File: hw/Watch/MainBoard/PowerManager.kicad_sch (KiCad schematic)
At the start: 4 parts, among them U4 LD39200

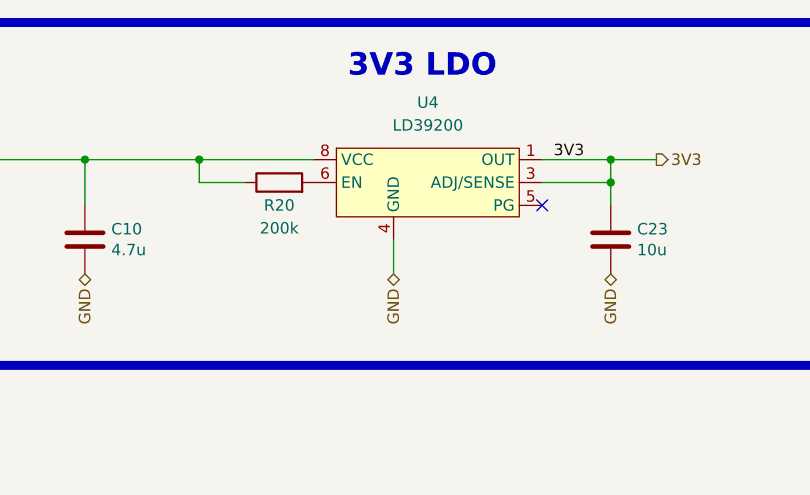
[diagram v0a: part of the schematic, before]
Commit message: wip
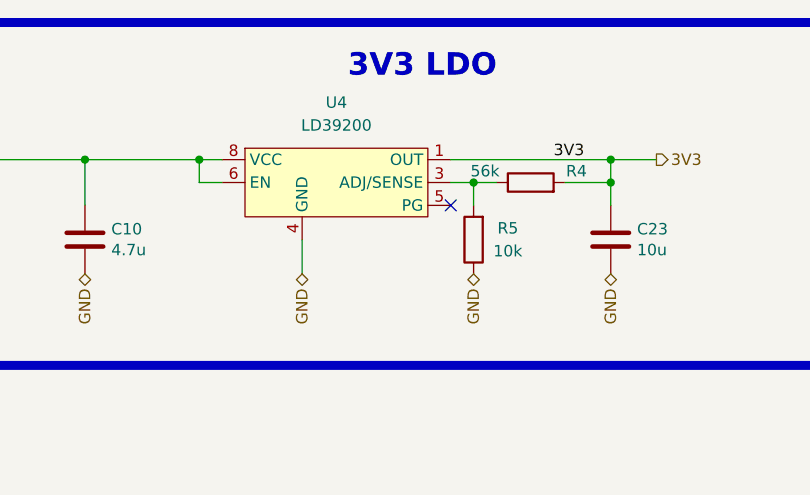
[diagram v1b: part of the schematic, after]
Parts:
- removed R20: 200k, Resistor_SMD:R_0402_1005Metric, symbol Device:R
- added R4: 56k, Resistor_SMD:R_0402_1005Metric, symbol Device:R
- added R5: 10k, Resistor_SMD:R_0201_0603Metric, symbol Device:R
- C10: footprint Capacitor_SMD:C_0603_1608Metric -> Capacitor_SMD:C_0402_1005Metric; LCSC C19666 -> C23733
- C23: footprint Capacitor_SMD:C_0603_1608Metric -> Capacitor_SMD:C_0402_1005Metric; Basic/Extended B -> E; LCSC C96446 -> C315248; info 25V, X5R -> 10V, X5R
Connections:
- net 3V3: now also R4.2; no longer U4.3 (ADJ/SENSE)
- net GND: now also R5.1
- net VCC: now also U4.6 (EN)
- new net: R4.1, R5.2, U4.3 (ADJ/SENSE)
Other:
- moved on the sheet: U4
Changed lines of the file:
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@@
   (junction (at 152.4 40.64) (diameter 0) (color 0 0 0 0)
   )
+  (junction (at 195.58 43.18) (diameter 0) (color 0 0 0 0)
+  )
   (junction (at 210.82 40.64) (diameter 0) (color 0 0 0 0)
   )
@@
   )
   (no_connect (at 137.16 129.54))
-  (no_connect (at 203.2 45.72))
+  (no_connect (at 193.04 45.72))
   (no_connect (at 137.16 127))
   (wire (pts (xy 210.82 43.18) (xy 210.82 40.64))
@@
     (stroke (width 0) (type default))
   )
-  (wire (pts (xy 203.2 40.64) (xy 210.82 40.64))
+  (wire (pts (xy 193.04 40.64) (xy 210.82 40.64))
+    (stroke (width 0) (type default))
+  )
+  (wire (pts (xy 195.58 43.18) (xy 198.12 43.18))
+    (stroke (width 0) (type default))
+  )
+  (wire (pts (xy 195.58 43.18) (xy 195.58 45.72))
     (stroke (width 0) (type default))
   )
@@
     (stroke (width 1) (type default))
   )
-  (wire (pts (xy 165.1 40.64) (xy 177.8 40.64))
+  (wire (pts (xy 165.1 40.64) (xy 167.64 40.64))
     (stroke (width 0) (type default))
   )
@@
     (stroke (width 0) (type default))
   )
-  (wire (pts (xy 186.69 49.53) (xy 186.69 53.34))
+  (wire (pts (xy 176.53 49.53) (xy 176.53 53.34))
     (stroke (width 0) (type default))
   )
@@
     (stroke (width 0) (type default))
   )
-  (wire (pts (xy 203.2 43.18) (xy 210.82 43.18))
-    (stroke (width 0) (type default))
-  )
-  (wire (pts (xy 170.18 43.18) (xy 165.1 43.18))
+  (wire (pts (xy 193.04 43.18) (xy 195.58 43.18))
+    (stroke (width 0) (type default))
+  )
+  (wire (pts (xy 165.1 43.18) (xy 167.64 43.18))
     (stroke (width 0) (type default))
   )
@@
   )
   (wire (pts (xy 104.14 73.66) (xy 101.6 73.66))
+    (stroke (width 0) (type default))
+  )
+  (wire (pts (xy 205.74 43.18) (xy 210.82 43.18))
     (stroke (width 0) (type default))
   )
@@
     (effects (font (size 1.27 1.27)) (justify left bottom))
   )
+  (hierarchical_label "GND" (shape bidirectional) (at 195.58 53.34 270) (fields_autoplaced)
+    (effects (font (size 1.27 1.27)) (justify right))
+  )
   (hierarchical_label "3V3" (shape output) (at 215.9 40.64 0) (fields_autoplaced)
     (effects (font (size 1.27 1.27)) (justify left))
@@
     (effects (font (size 1.27 1.27)) (justify right))
   )
-  (hierarchical_label "GND" (shape bidirectional) (at 186.69 53.34 270) (fields_autoplaced)
+  (hierarchical_label "GND" (shape bidirectional) (at 176.53 53.34 270) (fields_autoplaced)
     (effects (font (size 1.27 1.27)) (justify right))
   )
@@
       (effects (font (size 1.27 1.27)) (justify left))
     )
-    (property "Footprint" "Capacitor_SMD:C_0603_1608Metric" (at 211.7852 53.34 0)
+    (property "Footprint" "Capacitor_SMD:C_0402_1005Metric" (at 211.7852 53.34 0)
       (effects (font (size 1.27 1.27)) hide)
     )
@@
       (effects (font (size 1.27 1.27)) hide)
     )
-    (property "LCSC" "C96446" (at 210.82 49.53 0)
-      (effects (font (size 1.27 1.27)) hide)
-    )
-    (property "Basic/Extended" "B" (at 210.82 49.53 0)
-      (effects (font (size 1.27 1.27)) hide)
-    )
-    (property "info" "25V, X5R" (at 210.82 49.53 0)
+    (property "LCSC" "C315248" (at 210.82 49.53 0)
+      (effects (font (size 1.27 1.27)) hide)
+    )
+    (property "Basic/Extended" "E" (at 210.82 49.53 0)
+      (effects (font (size 1.27 1.27)) hide)
+    )
+    (property "info" "10V, X5R" (at 210.82 49.53 0)
       (effects (font (size 1.27 1.27)) hide)
     )
@@
       (effects (font (size 1.27 1.27)) (justify left))
     )
-    (property "Footprint" "Capacitor_SMD:C_0603_1608Metric" (at 153.3652 53.34 0)
+    (property "Footprint" "Capacitor_SMD:C_0402_1005Metric" (at 153.3652 53.34 0)
       (effects (font (size 1.27 1.27)) hide)
     )
@@
       (effects (font (size 1.27 1.27)) hide)
     )
-    (property "LCSC" "C19666" (at 152.4 49.53 0)
+    (property "LCSC" "C23733" (at 152.4 49.53 0)
       (effects (font (size 1.27 1.27)) hide)
     )
@@
     )
   )
-  (symbol (lib_id "Device:R") (at 173.99 43.18 90) (unit 1)
+  (symbol (lib_id "Device:R") (at 201.93 43.18 90) (unit 1)
     (in_bom yes) (on_board yes) (dnp no)
-    (property "Reference" "R20" (at 173.99 45.72 90)
-      (effects (font (size 1.27 1.27)))
-    )
-    (property "Value" "200k" (at 173.99 48.26 90)
-      (effects (font (size 1.27 1.27)))
-    )
-    (property "Footprint" "Resistor_SMD:R_0402_1005Metric" (at 173.99 44.958 90)
-      (effects (font (size 1.27 1.27)) hide)
-    )
-    (property "Datasheet" "~" (at 173.99 43.18 0)
-      (effects (font (size 1.27 1.27)) hide)
-    )
-    (property "LCSC" "C25764" (at 173.99 43.18 0)
-      (effects (font (size 1.27 1.27)) hide)
-    )
-    (property "Basic/Extended" "B" (at 173.99 43.18 0)
+    (property "Reference" "R4" (at 207.01 41.91 90)
+      (effects (font (size 1.27 1.27)))
+    )
+    (property "Value" "56k" (at 196.85 41.91 90)
+      (effects (font (size 1.27 1.27)))
+    )
+    (property "Footprint" "Resistor_SMD:R_0402_1005Metric" (at 201.93 44.958 90)
+      (effects (font (size 1.27 1.27)) hide)
+    )
+    (property "Datasheet" "~" (at 201.93 43.18 0)
+      (effects (font (size 1.27 1.27)) hide)
+    )
+    (property "LCSC" "C25796" (at 201.93 43.18 0)
       (effects (font (size 1.27 1.27)) hide)
     )
@@
       (project "Watch"
         (path "/1db6f6a7-b341-422f-8dcc-b4fd8e3ba0c0/7a0b441f-fb08-4406-ad74-ba91736d76e3/e51762e8-40da-4e3a-afe4-857a6428bc26"
-          (reference "R20") (unit 1)
-        )
-      )
-      (project "ZakladniElektronika"
-        (path "/99cd3e15-4eb6-4cbb-8726-789aedd3df15/c3b70d9b-0dcb-4344-9507-13ff5b4c000e/aae02708-da26-44dd-a602-660fbe003309/3940fef8-969a-4db4-8b0b-434b96d98566"
-          (reference "R50") (unit 1)
-        )
-      )
-      (project "RB3203"
-        (path "/dc7f8a41-3453-4df6-94dc-e94521e89591/9c917b4f-c6c7-4191-9aaa-f982c264da50/8773969d-b2cc-42c4-9a6d-35c6f165cf16/da5be375-027b-4f55-96f0-042c23671c4c"
-          (reference "U?") (unit 1)
-        )
-      )
-    )
-  )
-  (symbol (lib_id "RKL-LDO:LD39200") (at 190.5 40.64 0) (unit 1)
+          (reference "R4") (unit 1)
+        )
+      )
+      (project "SemiSemafor"
+        (path "/fb82d987-26cf-425e-8e99-22ecb59c8a96"
+          (reference "R11") (unit 1)
+        )
+      )
+    )
+  )
+  (symbol (lib_id "Device:R") (at 195.58 49.53 180) (unit 1)
+    (in_bom yes) (on_board yes) (dnp no)
+    (property "Reference" "R5" (at 199.39 48.26 0)
+      (effects (font (size 1.27 1.27)))
+    )
+    (property "Value" "10k" (at 199.39 50.8 0)
+      (effects (font (size 1.27 1.27)))
+    )
+    (property "Footprint" "Resistor_SMD:R_0201_0603Metric" (at 197.358 49.53 90)
+      (effects (font (size 1.27 1.27)) hide)
+    )
+    (property "Datasheet" "~" (at 195.58 49.53 0)
+      (effects (font (size 1.27 1.27)) hide)
+    )
+    (property "LCSC" "C106225" (at 195.58 49.53 0)
+      (effects (font (size 1.27 1.27)) hide)
+    )
+    (property "Basic/Extended" "E" (at 195.58 49.53 0)
+      (effects (font (size 1.27 1.27)) hide)
+    )
+    (pin "1")
+    (pin "2")
+    (instances
+      (project "Watch"
+        (path "/1db6f6a7-b341-422f-8dcc-b4fd8e3ba0c0/7a0b441f-fb08-4406-ad74-ba91736d76e3/e51762e8-40da-4e3a-afe4-857a6428bc26"
+          (reference "R5") (unit 1)
+        )
+      )
+      (project "SemiSemafor"
+        (path "/fb82d987-26cf-425e-8e99-22ecb59c8a96"
+          (reference "R10") (unit 1)
+        )
+      )
+    )
+  )
+  (symbol (lib_id "RKL-LDO:LD39200") (at 180.34 40.64 0) (unit 1)
     (in_bom yes) (on_board yes) (dnp no) (fields_autoplaced)
-    (property "Reference" "U4" (at 190.5 34.29 0)
-      (effects (font (size 1.27 1.27)))
-    )
-    (property "Value" "LD39200" (at 190.5 36.83 0)
-      (effects (font (size 1.27 1.27)))
-    )
-    (property "Footprint" "Package_DFN_QFN:DFN-8-1EP_4x4mm_P0.8mm_EP2.3x3.24mm" (at 190.5 33.02 0)
-      (effects (font (size 1.27 1.27)) hide)
-    )
-    (property "Datasheet" "https://datasheet.lcsc.com/lcsc/2010270935_STMicroelectronics-LD39200DPUR_C880590.pdf" (at 190.5 30.48 0)
-      (effects (font (size 1.27 1.27)) hide)
-    )
-    (property "LCSC" "C880590" (at 190.5 27.94 0)
-      (effects (font (size 1.27 1.27)) hide)
-    )
-    (property "Basic/Extended" "E" (at 190.5 40.64 0)
-      (effects (font (size 1.27 1.27)) hide)
-    )
-    (property "JLCPCB_CORRECTION" "0;0;-90" (at 190.5 40.64 0)
-      (effects (font (size 1.27 1.27)) hide)
-    )
+    (property "Reference" "U4" (at 180.34 34.29 0)
+      (effects (font (size 1.27 1.27)))
+    )
+    (property "Value" "LD39200" (at 180.34 36.83 0)
+      (effects (font (size 1.27 1.27)))
+    )
+    (property "Footprint" "Package_DFN_QFN:DFN-8-1EP_4x4mm_P0.8mm_EP2.3x3.24mm" (at 180.34 33.02 0)
+      (effects (font (size 1.27 1.27)) hide)
+    )
+    (property "Datasheet" "https://datasheet.lcsc.com/lcsc/2010270935_STMicroelectronics-LD39200DPUR_C880590.pdf" (at 180.34 30.48 0)
+      (effects (font (size 1.27 1.27)) hide)
+    )
+    (property "LCSC" "C880590" (at 180.34 27.94 0)
+      (effects (font (size 1.27 1.27)) hide)
+    )
+    (property "Basic/Extended" "E" (at 180.34 40.64 0)
+      (effects (font (size 1.27 1.27)) hide)
+    )
+    (property "JLCPCB_CORRECTION" "0;0;-90" (at 180.34 40.64 0)
+      (effects (font (size 1.27 1.27)) hide)
+    )

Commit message: PCB
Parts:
- R5: footprint Resistor_SMD:R_0201_0603Metric -> Resistor_SMD:R_0402_1005Metric; Basic/Extended E -> B; LCSC C106225 -> C25744
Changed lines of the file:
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@@
       (effects (font (size 1.27 1.27)))
     )
-    (property "Footprint" "Resistor_SMD:R_0201_0603Metric" (at 197.358 49.53 90)
+    (property "Footprint" "Resistor_SMD:R_0402_1005Metric" (at 197.358 49.53 90)
       (effects (font (size 1.27 1.27)) hide)
     )
@@
       (effects (font (size 1.27 1.27)) hide)
     )
-    (property "LCSC" "C106225" (at 195.58 49.53 0)
+    (property "LCSC" "C25744" (at 195.58 49.53 0)
       (effects (font (size 1.27 1.27)) hide)
     )
-    (property "Basic/Extended" "E" (at 195.58 49.53 0)
+    (property "Basic/Extended" "B" (at 195.58 49.53 0)
       (effects (font (size 1.27 1.27)) hide)
     )
